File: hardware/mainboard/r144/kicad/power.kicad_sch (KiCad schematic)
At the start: 47 parts, among them J1 1S LiPo PCM / PH-2, J8 External cell NTC / hand sold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, Q2 AO3401A, SW1 MK-12C03-G015, U3 BQ24072TRGTR, U4 TPS63802DLAR

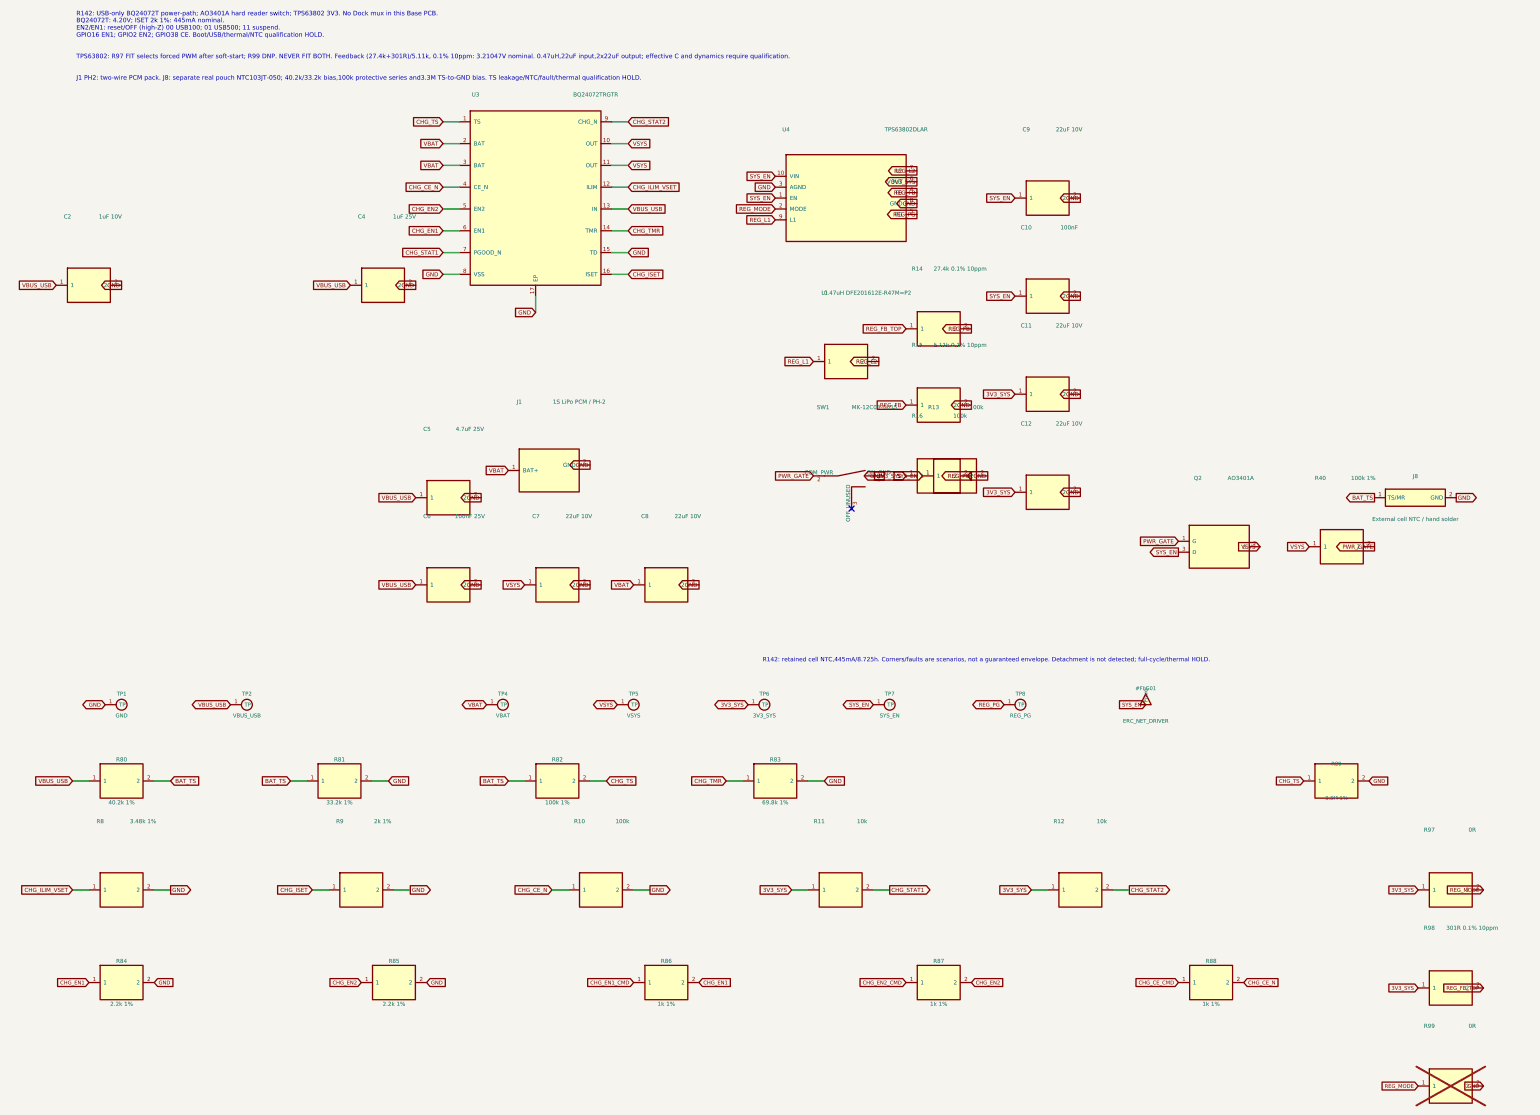
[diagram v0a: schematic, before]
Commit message: hardware(r144): route precision reset and PWM supply, fix rule compilation; native checks zero, independent review pending
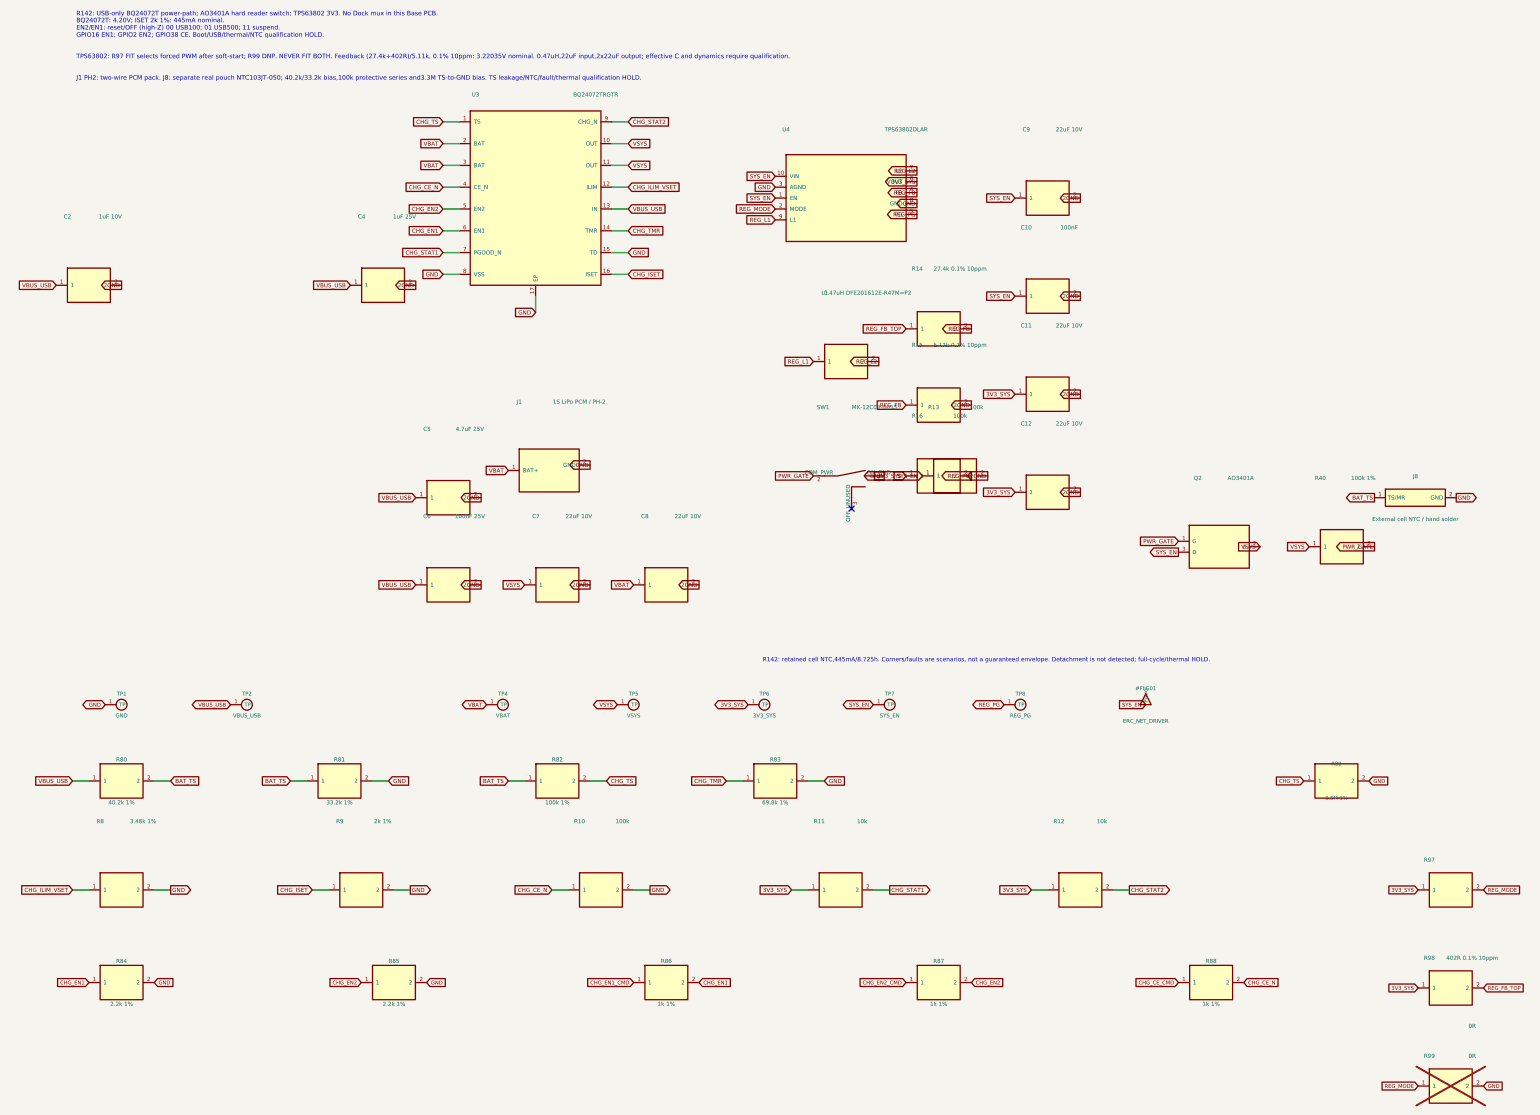
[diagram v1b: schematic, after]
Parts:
- R98: value 301R 0.1% 10ppm -> 402R 0.1% 10ppm; MPN RT0603BRB07301RL -> RT0603BRB07402RL
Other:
- note added: "TPS63802: R97 FIT selects forced PWM after soft-start; R99 DNP. NEVER FIT BOTH. Feedback (27.4k+402R)/5.11k, 0.1% 10ppm: 3.22035V nominal. 0.47uH,22uF input,2x22uF output; effective C and dynamics require qualification."
- note removed: "TPS63802: R97 FIT selects forced PWM after soft-start; R99 DNP. NEVER FIT BOTH. Feedback (27.4k+301R)/5.11k, 0.1% 10ppm: 3.21047V nominal. 0.47uH,22uF input,2x22uF output; effective C and dynamics require qualification."
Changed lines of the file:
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@@
 		(property "Footprint" "ENKU:R_RT0603_YAGEO_REFLOW" (at 226.06 92.71 0) (effects (font (size 0.95 0.95)) (hide yes)))
 		(property "Datasheet" "https://yageogroup.com/content/datasheet/asset/file/PYU-RT_1-TO-0-01_ROHS_L" (at 226.06 92.71 0) (effects (font (size 0.95 0.95)) (hide yes)))
-		(property "Description" "R144 upper feedback 27.4k plus R98 301R; PWM nominal 3.21047V" (at 226.06 92.71 0) (effects (font (size 0.95 0.95)) (hide yes)))
+		(property "Description" "R144 upper feedback 27.4k plus R98 402R; PWM nominal 3.22035V" (at 226.06 92.71 0) (effects (font (size 0.95 0.95)) (hide yes)))
 		(pin "1")
 		(pin "2")
@@
 		(property "Footprint" "ENKU:R_RT0603_YAGEO_REFLOW" (at 226.06 110.49 0) (effects (font (size 0.95 0.95)) (hide yes)))
 		(property "Datasheet" "https://yageogroup.com/content/datasheet/asset/file/PYU-RT_1-TO-0-01_ROHS_L" (at 226.06 110.49 0) (effects (font (size 0.95 0.95)) (hide yes)))
-		(property "Description" "R144 feedback bottom 5.11k; PWM nominal 3.21047V" (at 226.06 110.49 0) (effects (font (size 0.95 0.95)) (hide yes)))
+		(property "Description" "R144 feedback bottom 5.11k; PWM nominal 3.22035V" (at 226.06 110.49 0) (effects (font (size 0.95 0.95)) (hide yes)))
 		(pin "1")
 		(pin "2")
@@
 	(text "R142: USB-only BQ24072T power-path; AO3401A hard reader switch; TPS63802 3V3. No Dock mux in this Base PCB." (exclude_from_sim no) (at 25 20 0) (effects (font (size 1.05 1.05)) (justify left bottom)))
 	(text "BQ24072T: 4.20V; ISET 2k 1%: 445mA nominal.\nEN2/EN1: reset/OFF (high-Z) 00 USB100; 01 USB500; 11 suspend.\nGPIO16 EN1; GPIO2 EN2; GPIO38 CE. Boot/USB/thermal/NTC qualification HOLD." (exclude_from_sim no) (at 25 25 0) (effects (font (size 1.05 1.05)) (justify left bottom)))
-	(text "TPS63802: R97 FIT selects forced PWM after soft-start; R99 DNP. NEVER FIT BOTH. Feedback (27.4k+301R)/5.11k, 0.1% 10ppm: 3.21047V nominal. 0.47uH,22uF input,2x22uF output; effective C and dynamics require qualification." (exclude_from_sim no) (at 25 30 0) (effects (font (size 1.05 1.05)) (justify left bottom)))
+	(text "TPS63802: R97 FIT selects forced PWM after soft-start; R99 DNP. NEVER FIT BOTH. Feedback (27.4k+402R)/5.11k, 0.1% 10ppm: 3.22035V nominal. 0.47uH,22uF input,2x22uF output; effective C and dynamics require qualification." (exclude_from_sim no) (at 25 30 0) (effects (font (size 1.05 1.05)) (justify left bottom)))
 	(text "J1 PH2: two-wire PCM pack. J8: separate real pouch NTC103JT-050; 40.2k/33.2k bias,100k protective series and3.3M TS-to-GND bias. TS leakage/NTC/fault/thermal qualification HOLD." (exclude_from_sim no) (at 25 35 0) (effects (font (size 1.05 1.05)) (justify left bottom)))
 	(symbol (lib_id "ENKU:TESTPOINT") (at 35.56 180.34 0) (unit 1) (exclude_from_sim no) (in_bom no) (on_board yes) (dnp no)
@@
 (global_label "GND" (shape input) (at 326.390000 198.120000 180) (effects (font (size .88 .88)) (justify left bottom)))
 (symbol (lib_id "ENKU:R") (at 345.440000 223.520000 0) (unit 1) (exclude_from_sim no) (in_bom yes) (on_board yes) (dnp no)
-		(property "Reference" "R97" (at 340.440000 209.520000 0) (effects (font (size 0.95 0.95))))
-		(property "Value" "0R" (at 350.440000 209.520000 0) (effects (font (size 0.95 0.95))))
+		(property "Reference" "R97" (at 340.440000 216.520000 0) (effects (font (size 0.95 0.95))))
+		(property "Value" "0R" (at 350.440000 262.240000 0) (effects (font (size 0.95 0.95))))
 		(property "Footprint" "ENKU:R_RC0603_YAGEO_REFLOW" (at 345.440000 223.520000 0) (effects (font (size 0.95 0.95)) (hide yes)))
 		(property "Datasheet" "https://yageogroup.com/content/datasheet/asset/file/PYU-RC_GROUP_51_ROHS_L" (at 345.440000 223.520000 0) (effects (font (size 0.95 0.95)) (hide yes)))
@@
 )
 (global_label "3V3_SYS" (shape input) (at 337.820000 223.520000 0) (effects (font (size .88 .88)) (justify right bottom)))
-(global_label "REG_MODE" (shape input) (at 353.060000 223.520000 0) (effects (font (size .88 .88)) (justify right bottom)))
+(global_label "REG_MODE" (shape input) (at 353.060000 223.520000 180) (effects (font (size .88 .88)) (justify left bottom)))
 (symbol (lib_id "ENKU:R") (at 345.440000 246.380000 0) (unit 1) (exclude_from_sim no) (in_bom yes) (on_board yes) (dnp no)
-		(property "Reference" "R98" (at 340.440000 232.380000 0) (effects (font (size 0.95 0.95))))
-		(property "Value" "301R 0.1% 10ppm" (at 350.440000 232.380000 0) (effects (font (size 0.95 0.95))))
+		(property "Reference" "R98" (at 340.440000 239.380000 0) (effects (font (size 0.95 0.95))))
+		(property "Value" "402R 0.1% 10ppm" (at 350.440000 239.380000 0) (effects (font (size 0.95 0.95))))
 		(property "Footprint" "ENKU:R_RT0603_YAGEO_REFLOW" (at 345.440000 246.380000 0) (effects (font (size 0.95 0.95)) (hide yes)))
 		(property "Datasheet" "https://yageogroup.com/content/datasheet/asset/file/PYU-RT_1-TO-0-01_ROHS_L" (at 345.440000 246.380000 0) (effects (font (size 0.95 0.95)) (hide yes)))
@@
 		(pin "2")
 		(instances (project "enku-mainboard-r0.1" (path "/10000000-0000-4000-8000-000000000001/0398660f-aa9c-511d-bed1-18ce24e7f2f3" (reference "R98") (unit 1))))
-		(property "MPN" "RT0603BRB07301RL" (at 119.380000 135.890000 0) (effects (font (size .8 .8)) (hide yes)))
+		(property "MPN" "RT0603BRB07402RL" (at 119.380000 135.890000 0) (effects (font (size .8 .8)) (hide yes)))
 		(property "Manufacturer" "Yageo" (at 119.380000 135.890000 0) (effects (font (size .8 .8)) (hide yes)))
 		(property "Assembly" "FIT" (at 119.380000 135.890000 0) (effects (font (size .8 .8)) (hide yes)))
@@
 )
 (global_label "3V3_SYS" (shape input) (at 337.820000 246.380000 0) (effects (font (size .88 .88)) (justify right bottom)))
-(global_label "REG_FB_TOP" (shape input) (at 353.060000 246.380000 0) (effects (font (size .88 .88)) (justify right bottom)))
+(global_label "REG_FB_TOP" (shape input) (at 353.060000 246.380000 180) (effects (font (size .88 .88)) (justify left bottom)))
 (symbol (lib_id "ENKU:R") (at 345.440000 269.240000 0) (unit 1) (exclude_from_sim no) (in_bom yes) (on_board yes) (dnp yes)
-		(property "Reference" "R99" (at 340.440000 255.240000 0) (effects (font (size 0.95 0.95))))
+		(property "Reference" "R99" (at 340.440000 262.240000 0) (effects (font (size 0.95 0.95))))
 		(property "Value" "0R" (at 350.440000 255.240000 0) (effects (font (size 0.95 0.95))))
 		(property "Footprint" "ENKU:R_RC0603_YAGEO_REFLOW_DNP_NO_PASTE" (at 345.440000 269.240000 0) (effects (font (size 0.95 0.95)) (hide yes)))
@@
 )
 (global_label "REG_MODE" (shape input) (at 337.820000 269.240000 0) (effects (font (size .88 .88)) (justify right bottom)))
-(global_label "GND" (shape input) (at 353.060000 269.240000 0) (effects (font (size .88 .88)) (justify right bottom)))
-)
+(global_label "GND" (shape input) (at 353.060000 269.240000 180) (effects (font (size .88 .88)) (justify left bottom)))
+)
